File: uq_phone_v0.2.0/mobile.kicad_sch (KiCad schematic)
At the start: 29 parts, among them J10 513382474, J11 513382474, J12 20279-001E-03, J4 20279-001E-03, J5 20279-001E-03, U4 RC7620_1104626

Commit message: Cleaning up adn fixing massive mistake
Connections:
- net GND: now also J10.5, J10.6, J10.7, J10.8
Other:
- note added: "UQ Phone"
- note removed: "0.3A/contact"
- note removed: "Antenna"
- note removed: "Mobile Module"
- note removed: "Power Control"
- title: UQ Phone -> Mobile System
- moved on the sheet: J10, J11, J12, J4, J5

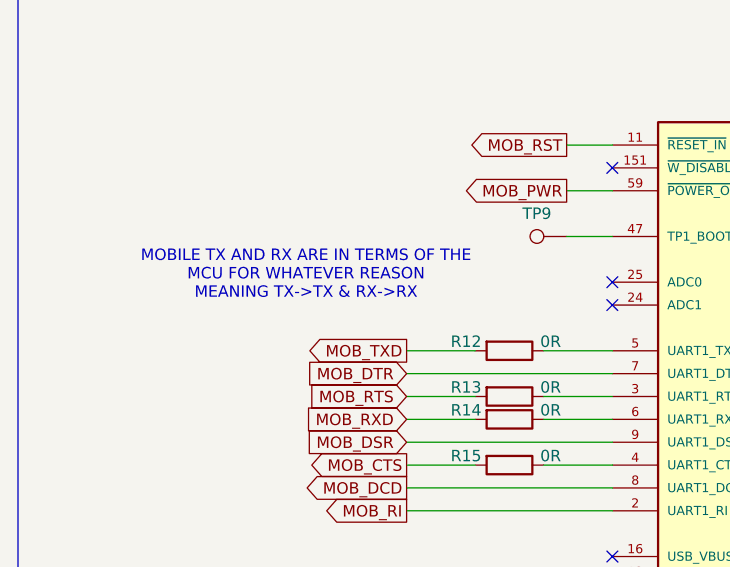
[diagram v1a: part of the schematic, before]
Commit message: minor comments
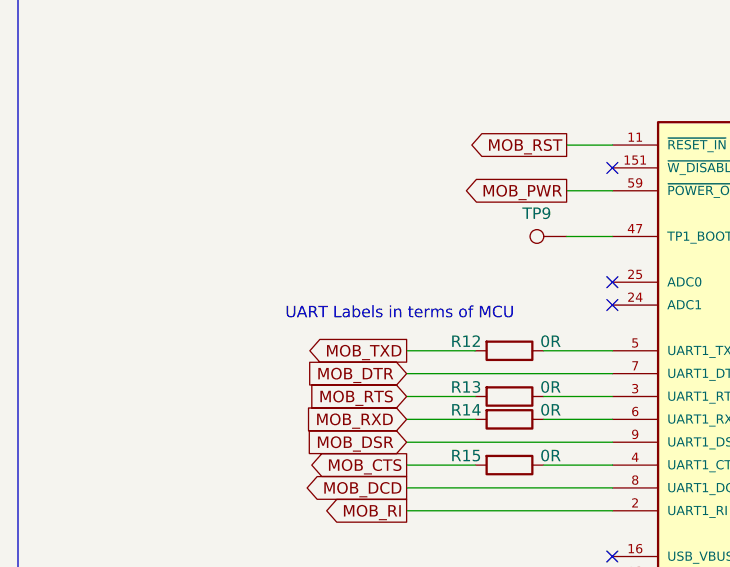
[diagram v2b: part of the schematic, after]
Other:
- note added: "UART Labels in terms of MCU"
- note removed: "MOBILE TX AND RX ARE IN TERMS OF THE MCU FOR WHATEVER REASON MEANING TX->TX & RX->RX"
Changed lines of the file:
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@@
 		)
 	)
-	(text "MOBILE TX AND RX ARE IN TERMS OF THE \nMCU FOR WHATEVER REASON \nMEANING TX->TX & RX->RX"
+	(text "UART Labels in terms of MCU"
 		(exclude_from_sim no)
-		(at 48.514 50.038 0)
+		(at 58.928 54.356 0)
 		(effects
 			(font
